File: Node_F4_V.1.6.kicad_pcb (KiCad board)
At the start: 2 copper layers, 97.5 x 59 mm, 178 parts, among them IC2 MP1584EN, J1 Conn_Jack-DC, J2 Conn_01x10, J3 Conn_01x16_Female, J4 RF_IPEX_U.FL-R-SMT, J5 SWD, J6 WiFi_Prog, J7 RS485, J8 LoRa_Anten, Q1 P_Mosfet, Q2 MMBT3904L, Q3 BC847, SW1 SW_Push, SW2 SW_Push, SW3 SW_Push, U1 SX1278, U2 SP3485EN, U3 STM32F407VETx, U4 Flash_W25Q128, U5 DS3231M, U6 ESP32-D0WD-V3, U7 W25Q128JVS, U8 MASWSS0192, Y1 8MHz, Y2 40MHz, Y3 32MHz

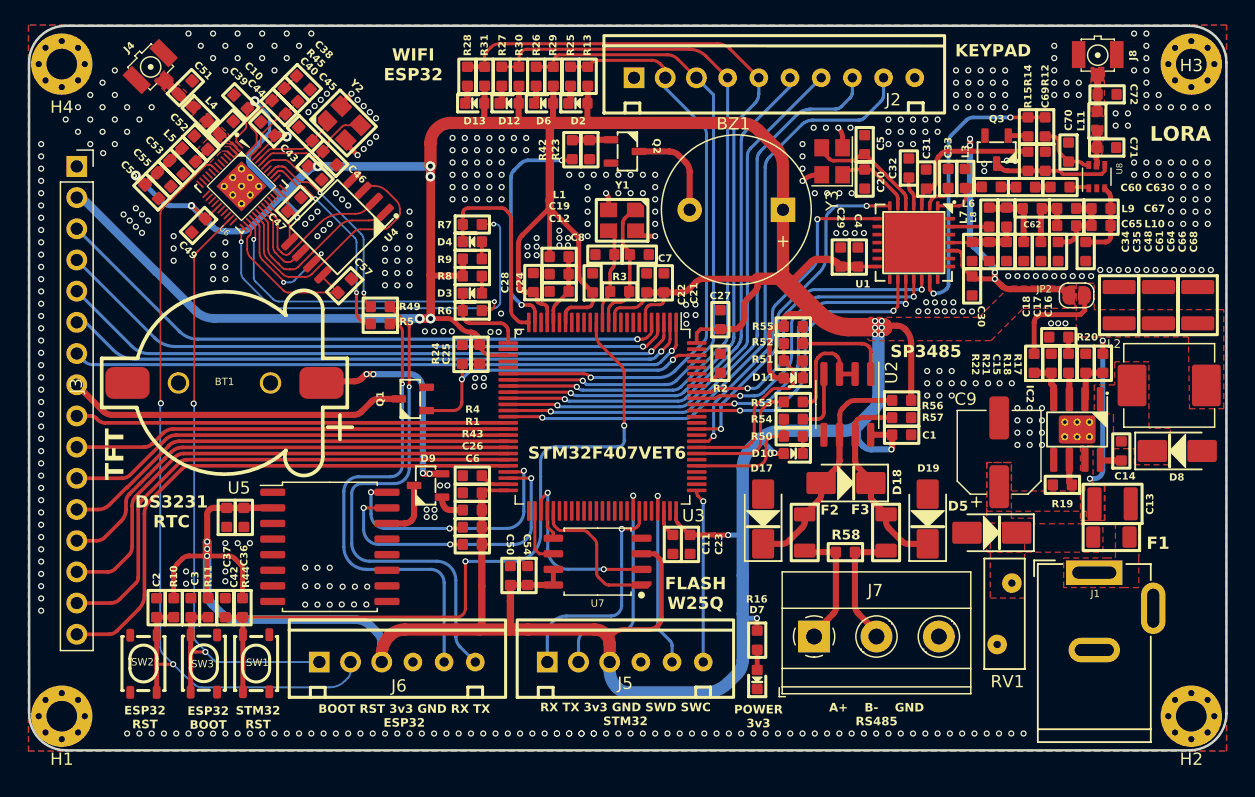
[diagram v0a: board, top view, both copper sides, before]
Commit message: Layout flash ESP32
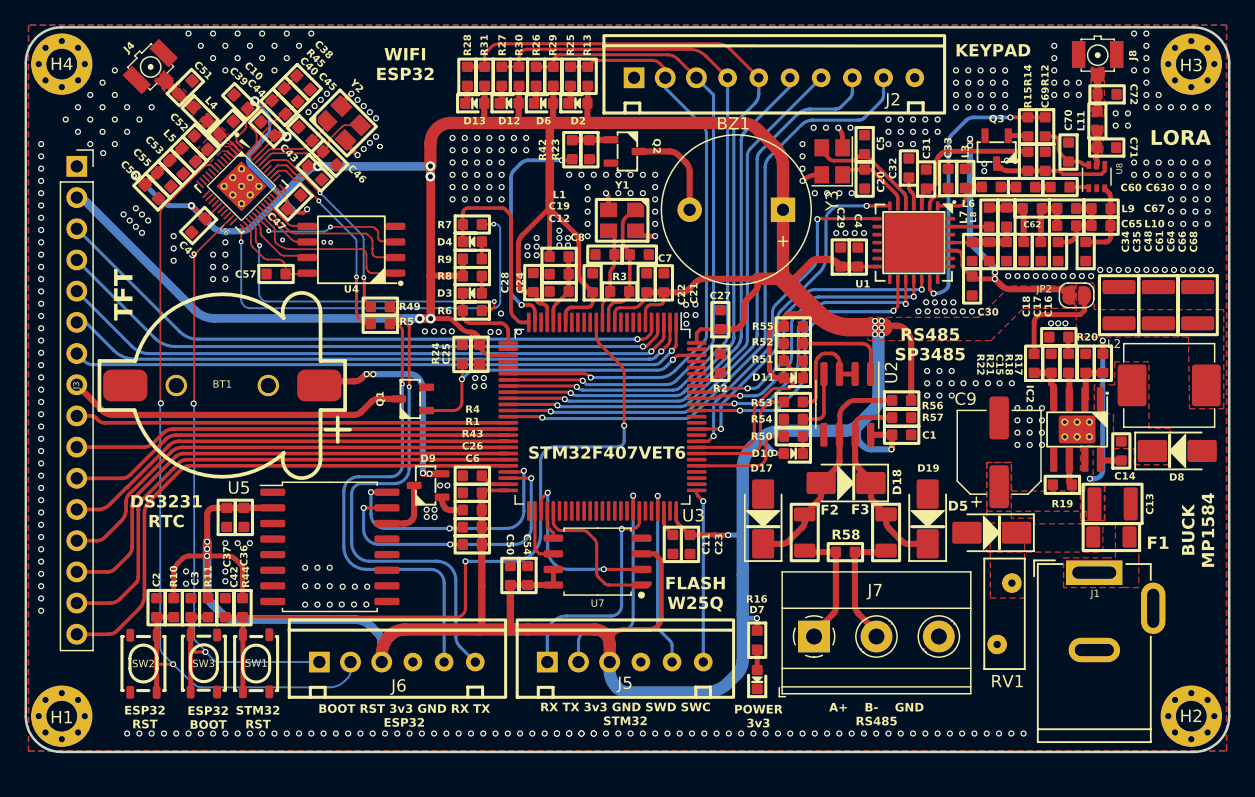
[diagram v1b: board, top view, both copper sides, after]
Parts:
- moved C57 5.67 mm to (93.1, 86.6), turned to 0 degrees
- moved U4 2.16 mm to (99.3, 84.6), turned to 180 degrees
- moved BT1 0.28 mm to (88.8, 95.7)
- moved C47 0.18 mm to (94.6, 80.7)
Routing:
- net /SWP_SD3: track 21.7 -> 13.0 mm, vias 0 -> 2
- net Net-(U4-VCC): track 13.2 -> 7.80 mm
- net /SHD_SD2: track 11.3 -> 6.11 mm, vias 2 -> 0
- net /SCK_CLK: track 6.58 -> 4.76 mm
- net Net-(U6-GPIO16): track 34.1 -> 35.3 mm
- net +3.3V: track 499.8 -> 501.0 mm
- net /SCS_CMD: track 15.5 -> 14.5 mm
- net GND: vias 492 -> 478
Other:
- board size 97.5 x 59 mm -> 98 x 59 mm
- board text added: "BUCK MP1584"
- board text added: "RS485 SP3485"
- board text removed: "SP3485"
